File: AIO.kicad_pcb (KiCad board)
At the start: 2 copper layers, 91 x 78 mm, 359 parts, among them J1 Conn_01x02_MountingPin, J1 JST SH1.0, J1 PH2.0, J1 SH1.0, J1 Sh 1.0, J2 SH1.0, J2 USB_C_Receptacle_PowerOnly_6P, J2 USB_C_Receptacle_USB2.0_16P, J3 JST PH2.0, J3 SH1.0, J3 USB_C_Receptacle_PowerOnly_6P, J3 USB_C_Receptacle_USB2.0_16P, Q1 AO3401A, Q2 AO3400A, Q2 MBT3904DW1, SW1 Boot, SW1 Reset, SW1 SW_Push, SW1 SW_SPDT, SW2 Boot, SW2 Reset, SW2 SW_Push, SW2 SW_SPDT, SW3 Boot, SW3 SW_Push_SPDT, SW3 SW_SPDT, SW3 SW_SPDT_312, U1 AP2112K-3.3, U1 MPU-6050, U1 TP4057, U1 XC6206P182MR, U2 AP2112K-3.3, U2 ESP32-S3-WROOM-1, U2 ESP32-WROOM-32U, U2 IP5306, U2 MPU-6050, U3 ESP32-C3-MINI-1, U3 ESP32C3_SuperMini, U3 MCP73831-2-OT, U3 ME6211C33M5, U3 MPU-9250, U4 AP2112K-3.3, U4 MCP73831-2-OT, U4 MPU-6050, U4 TP4057, U5 ESP32-S2, U5 XC6206P182MR, U6 MPU-9250, Y1 40MHz

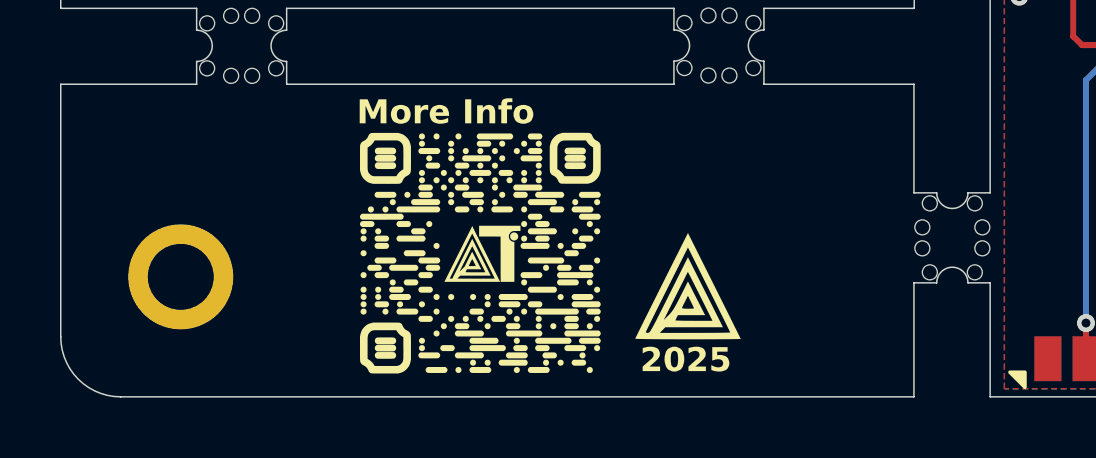
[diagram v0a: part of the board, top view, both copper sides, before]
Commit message: Update AIO.kicad_pcb
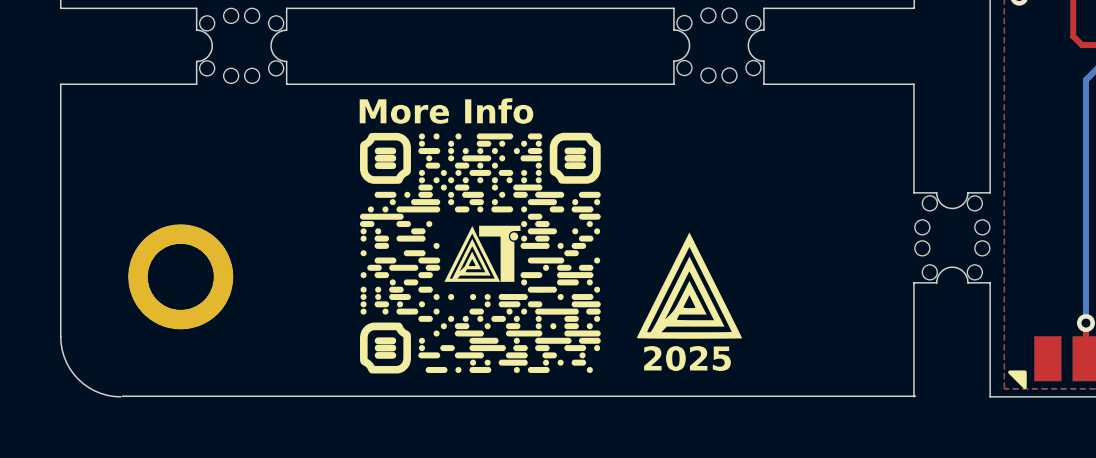
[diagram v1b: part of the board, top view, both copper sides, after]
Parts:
- moved G*** 0.05 mm to (192.4, 126.3)
- moved G*** 0.05 mm to (192.3, 126.3)
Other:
- outline, holes or cut-outs redrawn
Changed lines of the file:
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@@
 		(at 195.43 63.832019)
 		(property "Reference" "mouse-bite-1mm-slot"
-			(at 0 -2 360)
+			(at 0 -2 0)
 			(layer "F.SilkS")
 			(hide yes)
@@
 		)
 		(property "Value" "VAL**"
-			(at 0 2.1 360)
+			(at 0 2.1 0)
 			(layer "F.SilkS")
 			(hide yes)
@@
 		)
 		(property "Footprint" "Panelization Pretty:mouse-bite-1mm-slot"
-			(at 0 0 360)
+			(at 0 0 0)
 			(layer "F.Fab")
 			(hide yes)
@@
 		)
 		(property "Datasheet" ""
-			(at 0 0 360)
+			(at 0 0 0)
 			(layer "F.Fab")
 			(hide yes)
@@
 		)
 		(property "Description" ""
-			(at 0 0 360)
+			(at 0 0 0)
 			(layer "F.Fab")
 			(hide yes)
@@
 		(at 246.09096 118.5)
 		(property "Reference" "mouse-bite-1mm-slot"
-			(at 0 -2 360)
+			(at 0 -2 0)
 			(layer "F.SilkS")
 			(hide yes)
@@
 		)
 		(property "Value" "VAL**"
-			(at 0 2.1 360)
+			(at 0 2.1 0)
 			(layer "F.SilkS")
 			(hide yes)
@@
 		)
 		(property "Footprint" "Panelization Pretty:mouse-bite-1mm-slot"
-			(at 0 0 360)
+			(at 0 0 0)
 			(layer "F.Fab")
 			(hide yes)
@@
 		)
 		(property "Datasheet" ""
-			(at 0 0 360)
+			(at 0 0 0)
 			(layer "F.Fab")
 			(hide yes)
@@
 		)
 		(property "Description" ""
-			(at 0 0 360)
+			(at 0 0 0)
 			(layer "F.Fab")
 			(hide yes)
@@
 		(at 257.44 67.232019)
 		(property "Reference" "mouse-bite-1mm-slot"
-			(at 0 -2 360)
+			(at 0 -2 0)
 			(layer "F.SilkS")
 			(hide yes)
@@
 		)
 		(property "Value" "VAL**"
-			(at 0 2.1 360)
+			(at 0 2.1 0)
 			(layer "F.SilkS")
 			(hide yes)
@@
 		)
 		(property "Footprint" "Panelization Pretty:mouse-bite-1mm-slot"
-			(at 0 0 360)
+			(at 0 0 0)
 			(layer "F.Fab")
 			(hide yes)
@@
 		)
 		(property "Datasheet" ""
-			(at 0 0 360)
+			(at 0 0 0)
 			(layer "F.Fab")
 			(hide yes)
@@
 		)
 		(property "Description" ""
-			(at 0 0 360)
+			(at 0 0 0)
 			(layer "F.Fab")
 			(hide yes)
@@
 		(at 232.56 63.82952)
 		(property "Reference" "mouse-bite-1mm-slot"
-			(at 0 -2 360)
+			(at 0 -2 0)
 			(layer "F.SilkS")
 			(hide yes)
@@
 		)
 		(property "Value" "VAL**"
-			(at 0 2.1 360)
+			(at 0 2.1 0)
 			(layer "F.SilkS")
 			(hide yes)
@@
 		)
 		(property "Footprint" "Panelization Pretty:mouse-bite-1mm-slot"
-			(at 0 0 360)
+			(at 0 0 0)
 			(layer "F.Fab")
 			(hide yes)
@@
 		)
 		(property "Datasheet" ""
-			(at 0 0 360)
+			(at 0 0 0)
 			(layer "F.Fab")
 			(hide yes)
@@
 		)
 		(property "Description" ""
-			(at 0 0 360)
+			(at 0 0 0)
 			(layer "F.Fab")
 			(hide yes)
@@
 		(at 246.09096 67.232019)
 		(property "Reference" "mouse-bite-1mm-slot"
-			(at 0 -2 360)
+			(at 0 -2 0)
 			(layer "F.SilkS")
 			(hide yes)
@@
 		)
 		(property "Value" "VAL**"
-			(at 0 2.1 360)
+			(at 0 2.1 0)
 			(layer "F.SilkS")
 			(hide yes)
@@
 		)
 		(property "Footprint" "Panelization Pretty:mouse-bite-1mm-slot"
-			(at 0 0 360)
+			(at 0 0 0)
 			(layer "F.Fab")
 			(hide yes)
@@
 		)
 		(property "Datasheet" ""
-			(at 0 0 360)
+			(at 0 0 0)
 			(layer "F.Fab")
 			(hide yes)
@@
 		)
 		(property "Description" ""
-			(at 0 0 360)
+			(at 0 0 0)
 			(layer "F.Fab")
 			(hide yes)
@@
 		(at 222.8 63.832019)
 		(property "Reference" "mouse-bite-1mm-slot"
-			(at 0 -2 360)
+			(at 0 -2 0)
 			(layer "F.SilkS")
 			(hide yes)
@@
 		)
 		(property "Value" "VAL**"
-			(at 0 2.1 360)
+			(at 0 2.1 0)
 			(layer "F.SilkS")
 			(hide yes)
@@
 		)
 		(property "Footprint" "Panelization Pretty:mouse-bite-1mm-slot"
-			(at 0 0 360)
+			(at 0 0 0)
 			(layer "F.Fab")
 			(hide yes)
@@
 		)
 		(property "Datasheet" ""
-			(at 0 0 360)
+			(at 0 0 0)
 			(layer "F.Fab")
 			(hide yes)
@@
 		)
 		(property "Description" ""
-			(at 0 0 360)
+			(at 0 0 0)
 			(layer "F.Fab")
 			(hide yes)
@@
 	(footprint "LOGO"
 		(layer "F.Cu")
-		(at 192.32 126.36)
+		(at 192.37 126.34)
 		(property "Reference" "G***"
 			(at 0 0 0)
@@
 		(at 212.14 63.832019)
 		(property "Reference" "mouse-bite-1mm-slot"
-			(at 0 -2 360)
+			(at 0 -2 0)
 			(layer "F.SilkS")
 			(hide yes)
@@
 		)
 		(property "Value" "VAL**"
-			(at 0 2.1 360)
+			(at 0 2.1 0)
 			(layer "F.SilkS")
 			(hide yes)
@@
 		)
 		(property "Footprint" "Panelization Pretty:mouse-bite-1mm-slot"
-			(at 0 0 360)
+			(at 0 0 0)
 			(layer "F.Fab")
 			(hide yes)
@@
 		)
 		(property "Datasheet" ""
-			(at 0 0 360)
+			(at 0 0 0)
 			(layer "F.Fab")
 			(hide yes)
@@
 		)
 		(property "Description" ""
-			(at 0 0 360)
+			(at 0 0 0)
 			(layer "F.Fab")
 			(hide yes)
@@
 		(at 184.35 63.832019)
 		(property "Reference" "mouse-bite-1mm-slot"
-			(at 0 -2 360)
+			(at 0 -2 0)
 			(layer "F.SilkS")
 			(hide yes)
@@
 		)
 		(property "Value" "VAL**"
-			(at 0 2.1 360)
+			(at 0 2.1 0)
 			(layer "F.SilkS")
 			(hide yes)
@@
 		)
 		(property "Footprint" "Panelization Pretty:mouse-bite-1mm-slot"
-			(at 0 0 360)
+			(at 0 0 0)
 			(layer "F.Fab")
 			(hide yes)
@@
 		)
 		(property "Datasheet" ""
-			(at 0 0 360)
+			(at 0 0 0)
 			(layer "F.Fab")
 			(hide yes)
@@
 		)
 		(property "Description" ""
-			(at 0 0 360)
+			(at 0 0 0)
 			(layer "F.Fab")
 			(hide yes)
@@
 	(footprint "LOGO"
 		(layer "B.Cu")
-		(at 192.29 126.35 180)
+		(at 192.34 126.33 180)
 		(property "Reference" "G***"
 			(at 0 0 0)
@@
 	)
 	(gr_line
-		(start 173.4 130.13)
-		(end 199.84 130.13)
+		(start 173.45 130.11)
+		(end 199.89 130.11)
 		(stroke
 			(width 0.05)
@@
 	)
 	(gr_text "2025"
-		(at 193.9 129.36 -0)
+		(at 193.95 129.34 -0)
 		(layer "B.SilkS")
 		(effects
@@
 	)
 	(gr_text "2025"
-		(at 190.71 129.37 0)
+		(at 190.76 129.35 0)
 		(layer "F.SilkS")
 		(effects
